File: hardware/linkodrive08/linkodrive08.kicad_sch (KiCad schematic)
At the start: 103 parts, among them J1 USB_C_Receptacle_USB2.0_16P, J2 HALL, J3 WCH_SWD, J4 LKS_SWD, J5 MOT_POWER, J6 GATE_DRIVE, J7 LOGIC_POWER, J8 MOT, Q1 WSD4070DN, Q2 WSD4070DN, Q3 WSD4070DN, Q4 WSD4070DN, Q5 WSD4070DN, Q6 WSD4070DN, U1 LKS32MC086NxQx, U3 XL1509-ADJ, U4 TPS54260, U5 LGS5145, Y1 Crystal_GND24_Small

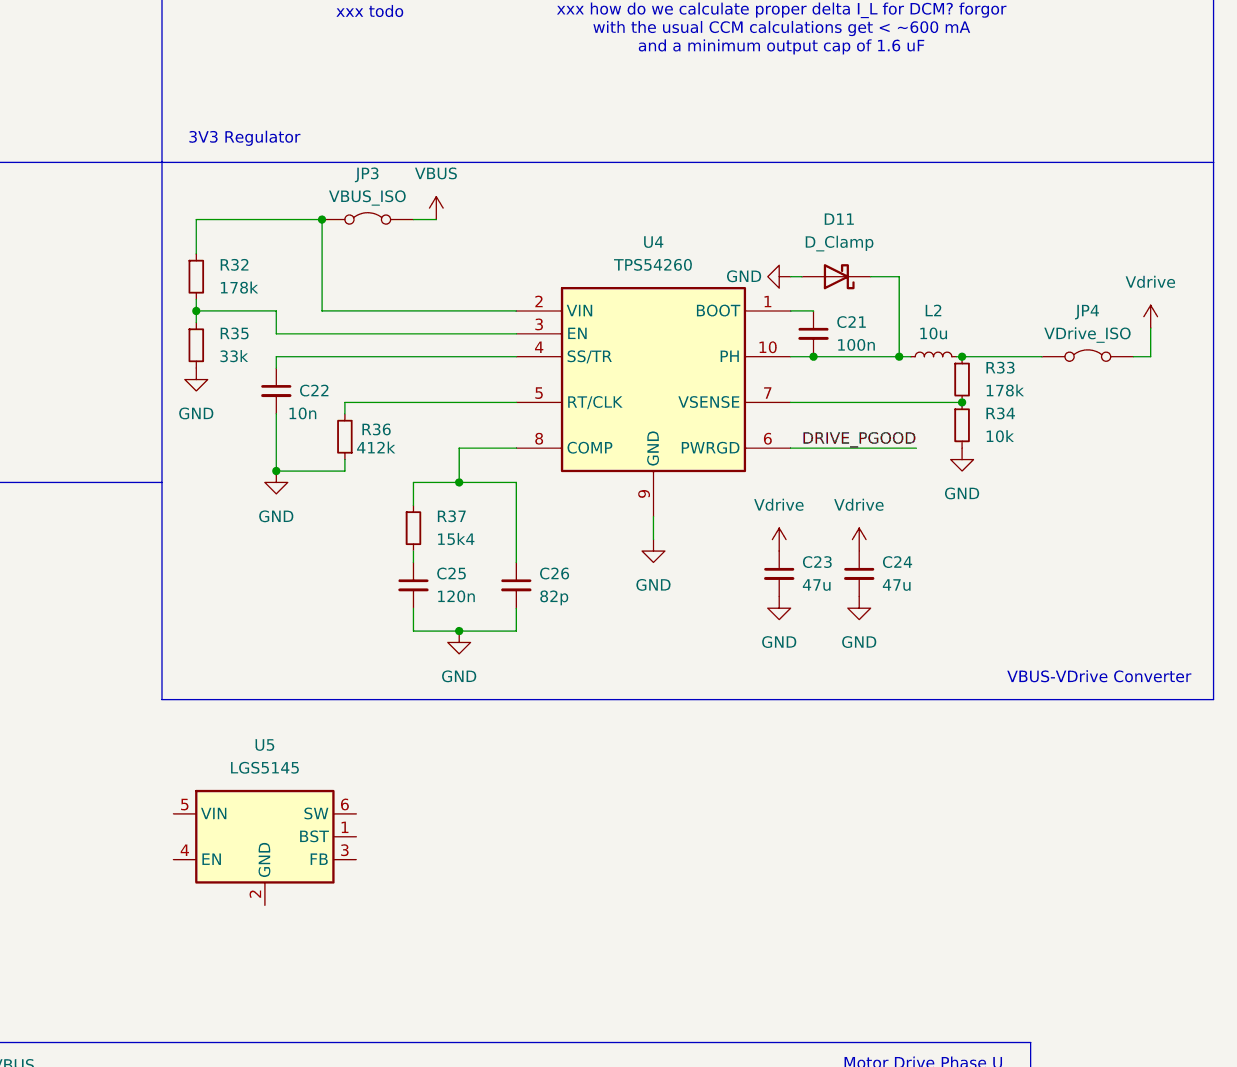
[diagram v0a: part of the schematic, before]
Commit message: work on design
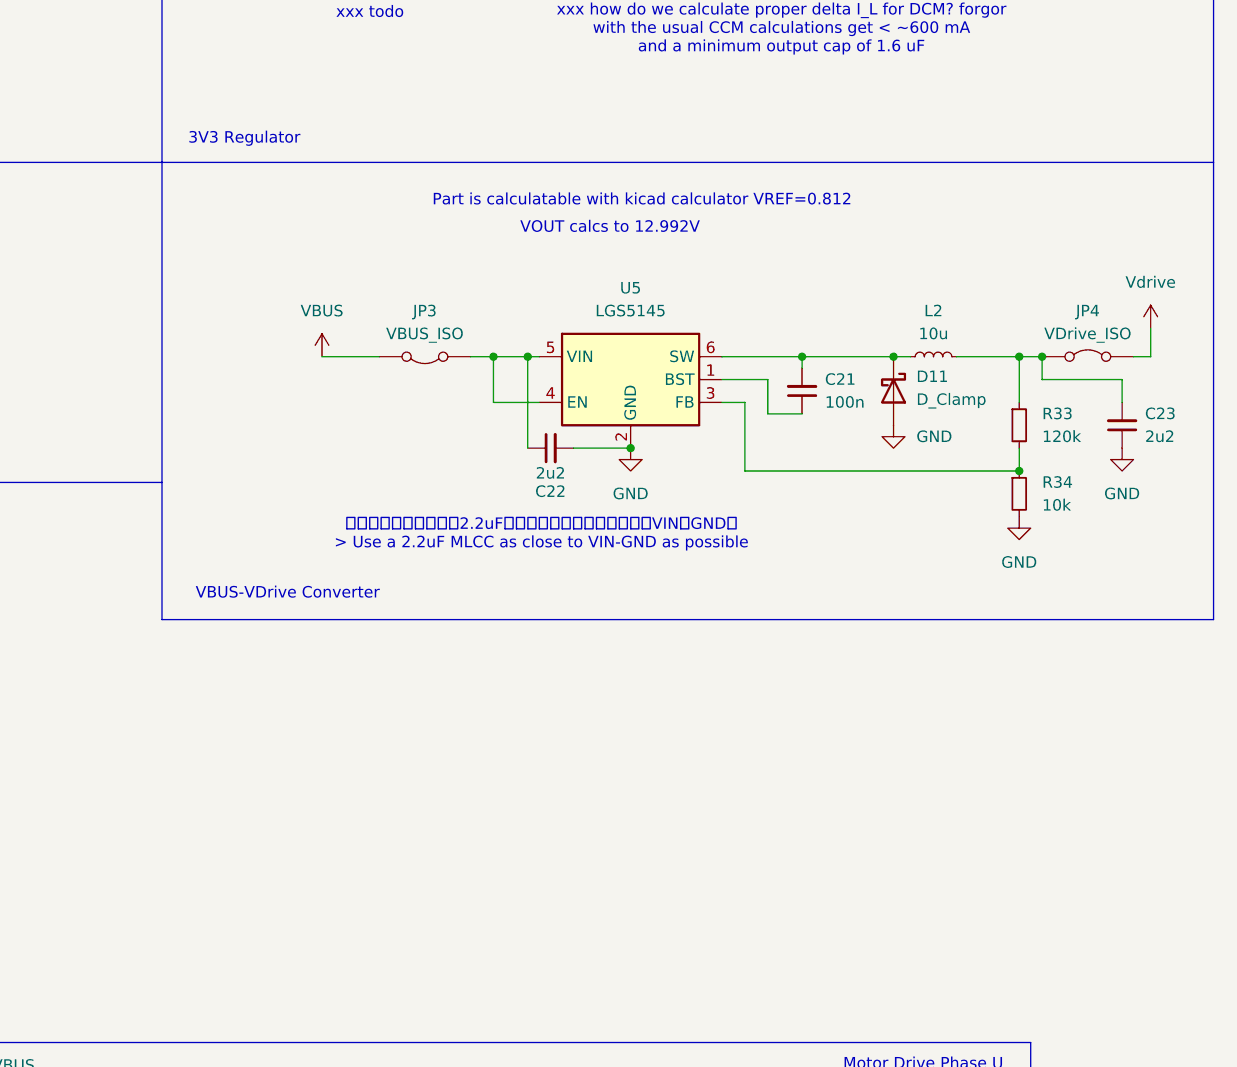
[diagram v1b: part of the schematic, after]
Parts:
- removed C24: 47u, symbol Device:C_Small
- removed C25: 120n, symbol Device:C_Small
- removed C26: 82p, symbol Device:C_Small
- removed R32: 178k, symbol Device:R_Small
- removed R35: 33k, symbol Device:R_Small
- removed R36: 412k, symbol Device:R_Small
- removed R37: 15k4, symbol Device:R_Small
- removed U4: TPS54260, Package_SO:MSOP-10-1EP_3x3mm_P0.5mm_EP1.68x1.88mm, symbol Missing_Symbols:TPS54260
- C22: value 10n -> 2u2
- C23: value 47u -> 2u2
- R33: value 178k -> 120k
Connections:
- net GND: now also C23.1, U5.2 (GND); no longer C23.2
- net Vdrive: no longer C23.1
- net at JP3.1 (A): now also C22.1, U5.4 (EN), U5.5 (VIN)
- net at C21.1: now also U5.1 (BST)
- net at C21.2, D11.1 (K), L2.1: now also U5.6 (SW)
- net at R33.2, R34.1: now also U5.3 (FB)
- net at JP4.1 (A), L2.2, R33.1: now also C23.2
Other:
- note added: "Part is calculatable with kicad calculator VREF=0.812"
- note added: "VOUT calcs to 12.992V"
- note added: "稳压器电源输入。使用2.2uF或更大的陶瓷贴片尽量近旁路VIN至GND。 > Use a 2.2uF MLCC as close to VIN-GND as possible"
- moved on the sheet: C21, D11, JP3, R33, R34, U5
